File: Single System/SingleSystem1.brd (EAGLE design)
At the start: 170 x 110 mm, 43 parts, among them U1 LMZ14203, U2 SD_CARD_SOCKET, U3 XBEE

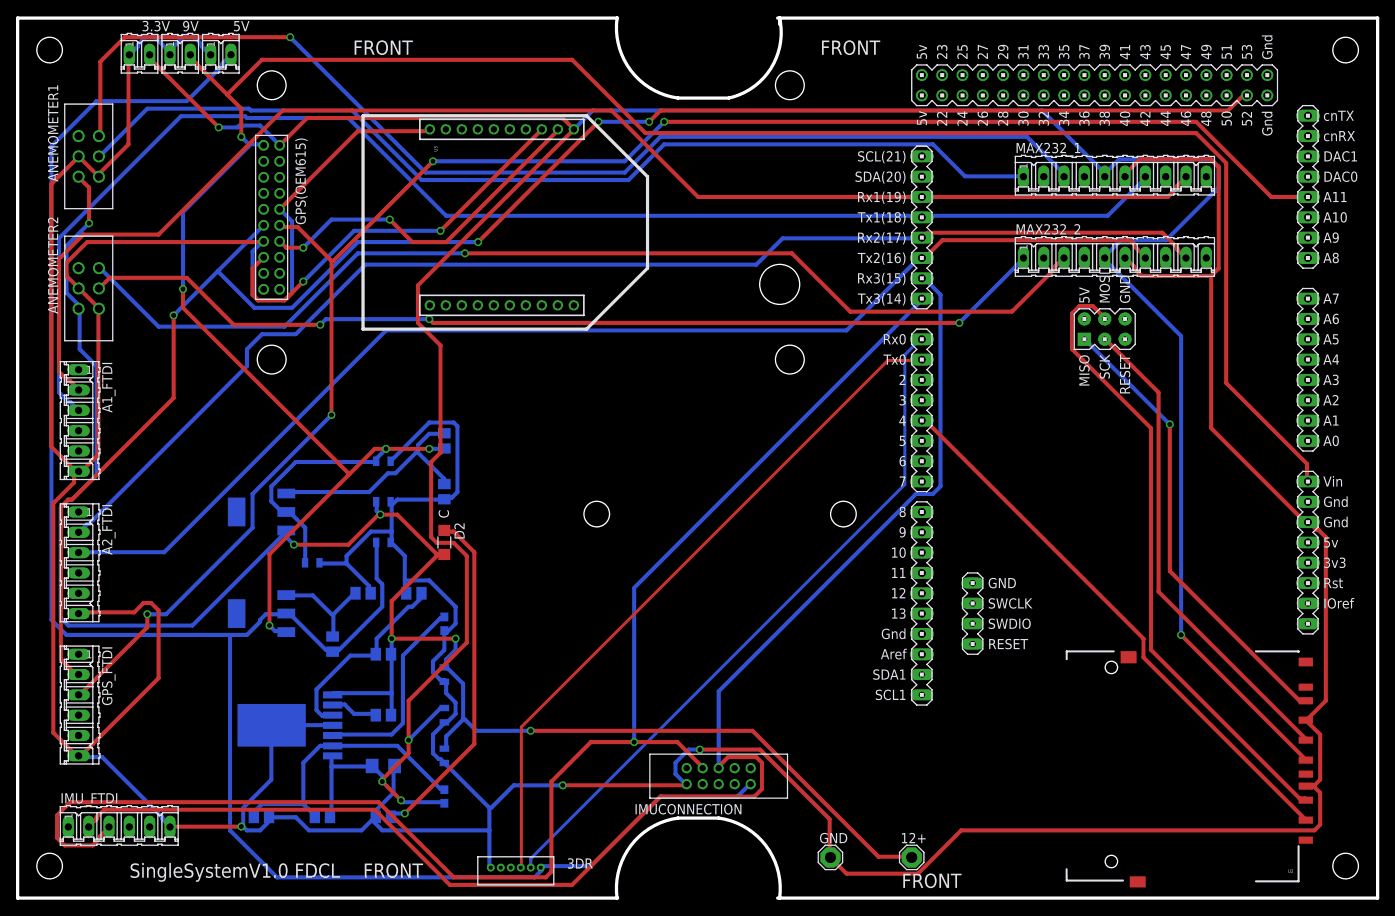
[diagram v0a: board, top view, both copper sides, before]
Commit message: final done
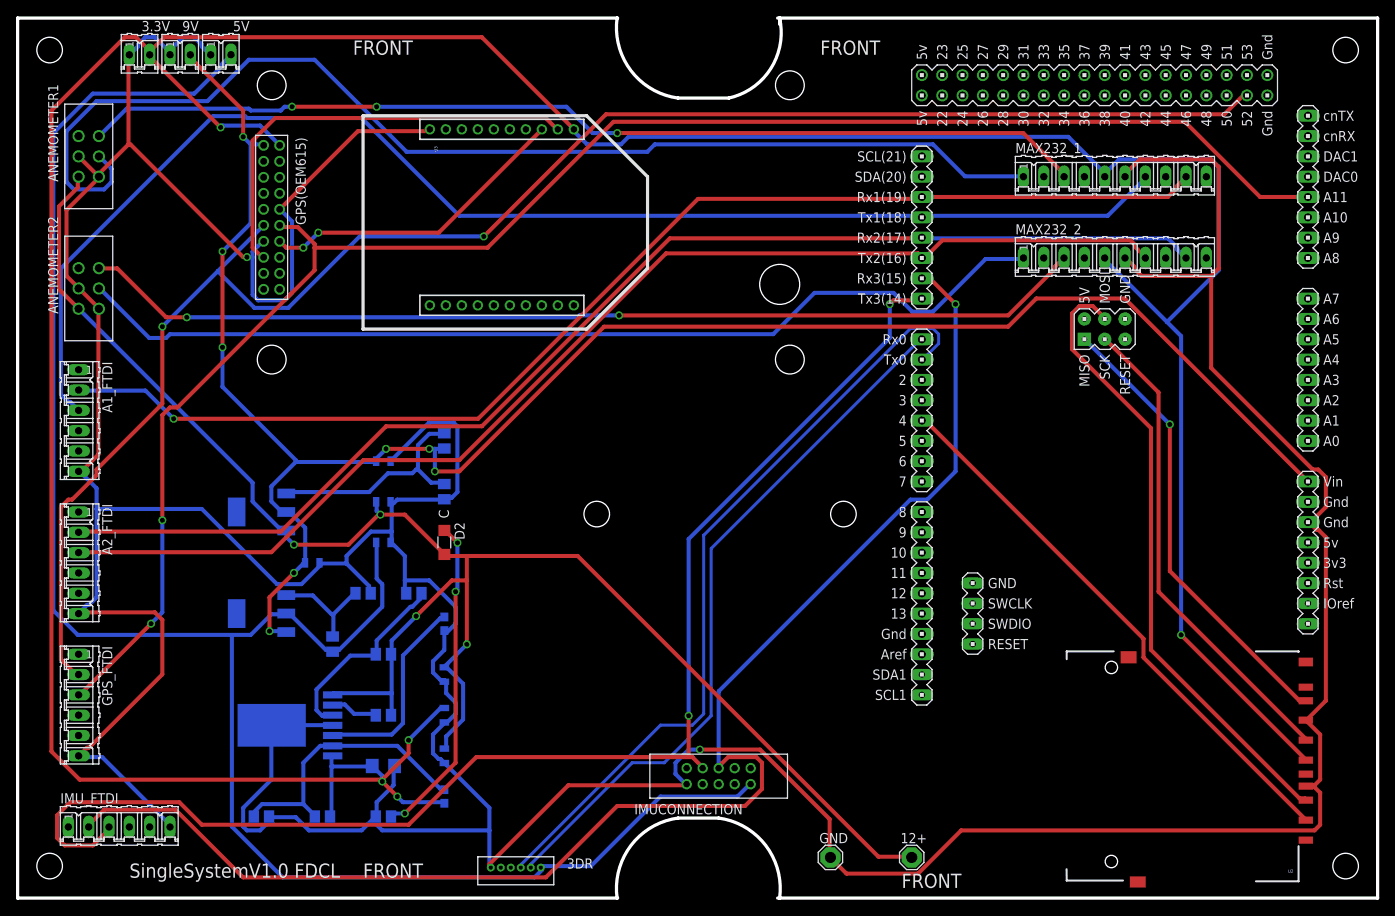
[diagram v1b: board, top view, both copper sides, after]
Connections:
- net XBEE_RX: now also U3.2; no longer U3.3
- net XBEE_TX: now also U3.3; no longer U3.2
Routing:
- net +9V: track 312.8 -> 239.9 mm, vias 5 -> 8
- net 3.3V: track 370.1 -> 438.7 mm
- net GND: track 685.0 -> 660.2 mm, vias 3 -> 2
- net +12V: track 238.3 -> 214.7 mm, vias 6 -> 4
- net A1_IN_TX: track 125.3 -> 146.8 mm
- net A1_RX: track 171.8 -> 152.7 mm, vias 0 -> 1
- net A1_IN_RX: track 142.3 -> 126.2 mm, vias 1 -> 3
- net IMU_RX: track 181.4 -> 169.0 mm, vias 1 -> 2
- net 3DR_RX: track 86.7 -> 97.8 mm
- net A2_IN_RX: track 133.4 -> 126.4 mm, vias 1 -> 2
- net XBEE_RX: track 50.6 -> 55.2 mm, vias 2 -> 0
- net XBEE_TX: track 43.6 -> 39.2 mm
- net A1_TX: track 172.3 -> 169.8 mm
- net 3DR_TX: track 86.6 -> 89.0 mm
- net N$7: track 43.1 -> 40.8 mm, vias 1 -> 3
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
